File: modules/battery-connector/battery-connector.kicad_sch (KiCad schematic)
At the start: 2 parts, among them J1 691210910002

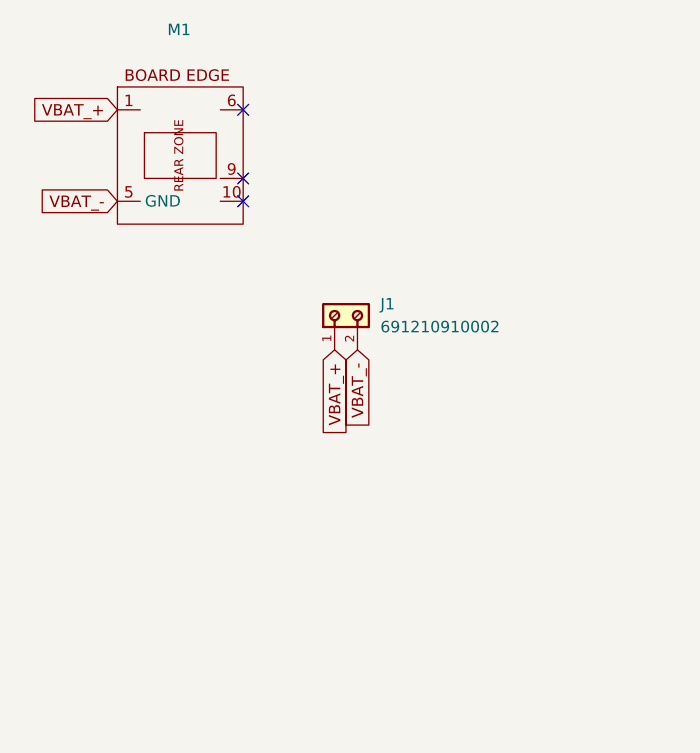
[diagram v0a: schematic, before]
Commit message: Updating all modules
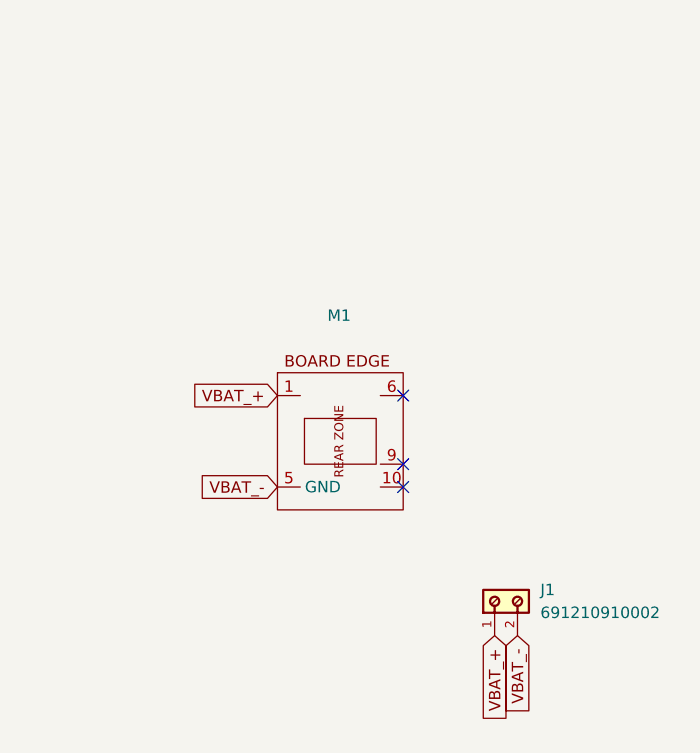
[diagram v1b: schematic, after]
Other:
- moved on the sheet: J1, M1
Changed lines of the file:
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@@
 	(paper "A4")
 	(no_connect
-		(at 119.38 59.69)
+		(at 137.16 91.44)
 	)
 	(no_connect
-		(at 119.38 52.07)
+		(at 137.16 83.82)
 	)
 	(no_connect
-		(at 119.38 62.23)
+		(at 137.16 93.98)
 	)
 	(global_label "VBAT_+"
 		(shape input)
-		(at 105.41 52.07 180)
+		(at 123.19 83.82 180)
 		(fields_autoplaced yes)
 		(effects
@@
 		)
 		(property "Intersheetrefs" "${INTERSHEET_REFS}"
-			(at 95.47 52.07 0)
+			(at 113.25 83.82 0)
 			(effects
 				(font
@@
 	(global_label "VBAT_-"
 		(shape input)
-		(at 105.41 62.23 180)
+		(at 123.19 93.98 180)
 		(fields_autoplaced yes)
 		(effects
@@
 		)
 		(property "Intersheetrefs" "${INTERSHEET_REFS}"
-			(at 95.47 62.23 0)
+			(at 113.25 93.98 0)
 			(effects
 				(font
@@
 	(global_label "VBAT_-"
 		(shape input)
-		(at 132.08 78.74 270)
+		(at 149.86 110.49 270)
 		(fields_autoplaced yes)
 		(effects
@@
 		)
 		(property "Intersheetrefs" "${INTERSHEET_REFS}"
-			(at 132.08 88.68 90)
+			(at 149.86 120.43 90)
 			(effects
 				(font
@@
 	(global_label "VBAT_+"
 		(shape input)
-		(at 129.54 78.74 270)
+		(at 147.32 110.49 270)
 		(fields_autoplaced yes)
 		(effects
@@
 		)
 		(property "Intersheetrefs" "${INTERSHEET_REFS}"
-			(at 129.54 88.68 90)
+			(at 147.32 120.43 90)
 			(effects
 				(font
@@
 	(symbol
 		(lib_id "MegaCastle:MegaCastle2x5-Module-I7.0x7.9-M8CC-EDGE")
-		(at 111.76 57.15 0)
+		(at 129.54 88.9 0)
 		(unit 1)
 		(exclude_from_sim no)
@@
 		(fields_autoplaced yes)
 		(property "Reference" "M1"
-			(at 112.2638 43.18 0)
+			(at 130.0438 74.93 0)
 			(effects
 				(font
@@
 		)
 		(property "Value" "~"
-			(at 112.2638 45.72 0)
+			(at 130.0438 77.47 0)
 			(effects
 				(font
@@
 		)
 		(property "Footprint" "MegaCastle:MegaCastle2x5-Module-I15.0x7.9-M8CC-SPAREPAD"
-			(at 111.76 69.85 0)
+			(at 129.54 101.6 0)
 			(effects
 				(font
@@
 		)
 		(property "Datasheet" ""
-			(at 111.76 52.07 0)
+			(at 129.54 83.82 0)
 			(effects
 				(font
@@
 		)
 		(property "Description" "Generated using footprint-gen .. 7 8 5 M8CC"
-			(at 111.76 57.15 0)
+			(at 129.54 88.9 0)
 			(effects
 				(font
@@
 	(symbol
 		(lib_id "691210910002:691210910002")
-		(at 132.08 73.66 0)
+		(at 149.86 105.41 0)
 		(unit 1)
 		(exclude_from_sim no)
@@
 		(fields_autoplaced yes)
 		(property "Reference" "J1"
-			(at 134.62 73.6599 0)
+			(at 152.4 105.4099 0)
 			(effects
 				(font
@@
 		)
 		(property "Value" "691210910002"
-			(at 134.62 76.1999 0)
+			(at 152.4 107.9499 0)
 			(effects
 				(font
@@
 		)
 		(property "Footprint" "MegaCastle:691210910002"
-			(at 132.08 73.66 0)
+			(at 149.86 105.41 0)
 			(effects
 				(font
@@
 		)
 		(property "Datasheet" ""
-			(at 132.08 73.66 0)
+			(at 149.86 105.41 0)
 			(effects
 				(font
@@
 		)
 		(property "Description" ""
-			(at 132.08 73.66 0)
+			(at 149.86 105.41 0)
 			(effects
 				(font
@@
 		)
 		(property "WIRE" "30 to 18 (AWG) 0.0509 to 0.823 (mm²)"
-			(at 132.08 73.66 0)
+			(at 149.86 105.41 0)
 			(effects
 				(font
@@
 		)
 		(property "MOUNT" "THT"
-			(at 132.08 73.66 0)
+			(at 149.86 105.41 0)
 			(effects
 				(font
@@
 		)
 		(property "IR-UL" "6A"
-			(at 132.08 73.66 0)
+			(at 149.86 105.41 0)
 			(effects
 				(font
@@
 		)
 		(property "WORKING-VOLTAGE-UL" "150V (AC)"
-			(at 132.08 73.66 0)
+			(at 149.86 105.41 0)
 			(effects
 				(font
@@
 		)
 		(property "PART-NUMBER" "691210910002"
-			(at 132.08 73.66 0)
+			(at 149.86 105.41 0)
 			(effects
 				(font
@@
 		)
 		(property "DATASHEET-URL" "https://www.we-online.com/redexpert/spec/691210910002?ae"
-			(at 132.08 73.66 0)
+			(at 149.86 105.41 0)
 			(effects
 				(font
@@
 		)
 		(property "PITCH" "2.54mm"
-			(at 132.08 73.66 0)
+			(at 149.86 105.41 0)
 			(effects
 				(font
@@
 		)
 		(property "PINS" "2"
-			(at 132.08 73.66 0)
+			(at 149.86 105.41 0)
 			(effects
 				(font
@@
 		)
 		(property "TYPE" "Horizontal"
-			(at 132.08 73.66 0)
-			(effects
-				(font
+			(at 149.86 105.41 0)
+			(effects
+				(font
